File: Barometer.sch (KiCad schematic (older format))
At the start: 5 parts, among them U9 BMP388

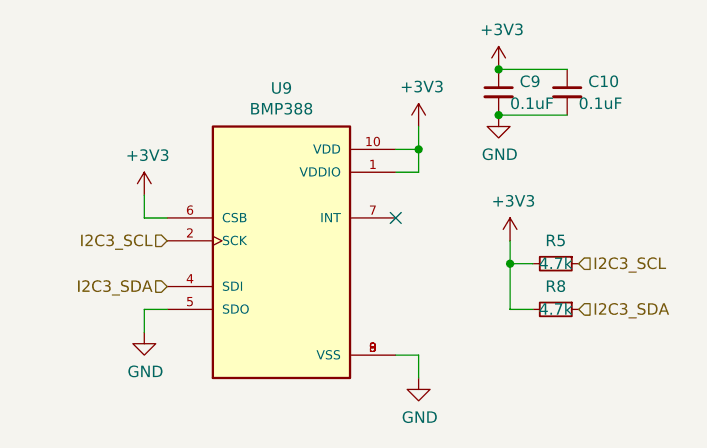
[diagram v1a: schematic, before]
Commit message: Changes made
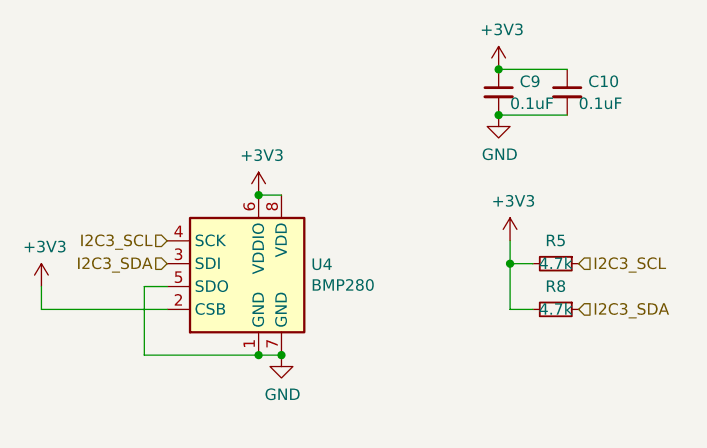
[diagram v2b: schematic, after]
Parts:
- removed U9: BMP388, Footprints:BMP388, symbol JPW_Symbols:BMP388
- added U4: BMP280, Package_LGA:Bosch_LGA-8_2x2.5mm_P0.65mm_ClockwisePinNumbering, symbol Sensor_Pressure:BMP280
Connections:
- net +3V3: now also U4.2 (CSB), U4.6 (VDDIO), U4.8 (VDD)
- net GND: now also U4.1 (GND), U4.5 (SDO), U4.7 (GND)
- net I2C3_SCL: now also U4.4 (SCK)
- net I2C3_SDA: now also U4.3 (SDI)
- no-connect marks 1 -> 0
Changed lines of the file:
@@
 $Descr A4 11693 8268
 encoding utf-8
-Sheet 7 7
+Sheet 5 7
 Title ""
 Date ""
@@
 Comment4 ""
 $EndDescr
-Text HLabel 5650 3950 0    50   Input ~ 0
+Text HLabel 5650 3850 0    50   Input ~ 0
 I2C3_SDA
 Text HLabel 5650 3750 0    50   Input ~ 0
 I2C3_SCL
 $Comp
-L JPW_Symbols:BMP388 U9
-U 1 1 608E517F
-P 6150 3850
-F 0 "U9" H 6150 4617 50  0000 C CNN
-F 1 "BMP388" H 6150 4526 50  0000 C CNN
-F 2 "Footprints:BMP388" H 6150 4600 50  0001 L BNN
-F 3 "" H 6150 3850 50  0001 L BNN
-	1    6150 3850
+L power:+3V3 #PWR0110
+U 1 1 608E9117
+P 6050 3550
+F 0 "#PWR0110" H 6050 3400 50  0001 C CNN
+F 1 "+3V3" H 6065 3723 50  0000 C CNN
+F 2 "" H 6050 3550 50  0001 C CNN
+F 3 "" H 6050 3550 50  0001 C CNN
+	1    6050 3550
 	1    0    0    -1
 $EndComp
 $Comp
-L power:+3V3 #PWR0110
-U 1 1 608E9117
-P 6750 3250
-F 0 "#PWR0110" H 6750 3100 50  0001 C CNN
-F 1 "+3V3" H 6765 3423 50  0000 C CNN
-F 2 "" H 6750 3250 50  0001 C CNN
-F 3 "" H 6750 3250 50  0001 C CNN
-	1    6750 3250
+L power:GND #PWR0171
+U 1 1 608EAE19
+P 6150 4250
+F 0 "#PWR0171" H 6150 4000 50  0001 C CNN
+F 1 "GND" H 6155 4077 50  0000 C CNN
+F 2 "" H 6150 4250 50  0001 C CNN
+F 3 "" H 6150 4250 50  0001 C CNN
+	1    6150 4250
 	1    0    0    -1
 $EndComp
 Wire Wire Line
-	6650 3350 6750 3350
-Wire Wire Line
-	6750 3350 6750 3250
-Wire Wire Line
-	6750 3350 6750 3450
-Wire Wire Line
-	6750 3450 6650 3450
-Connection ~ 6750 3350
-$Comp
-L power:+3V3 #PWR0111
-U 1 1 608E9B71
-P 5550 3550
-F 0 "#PWR0111" H 5550 3400 50  0001 C CNN
-F 1 "+3V3" H 5565 3723 50  0000 C CNN
-F 2 "" H 5550 3550 50  0001 C CNN
-F 3 "" H 5550 3550 50  0001 C CNN
-	1    5550 3550
-	1    0    0    -1
-$EndComp
-Wire Wire Line
-	5550 3550 5550 3650
-Wire Wire Line
-	5550 3650 5650 3650
-$Comp
-L power:GND #PWR0170
-U 1 1 608EA4FC
-P 5550 4150
-F 0 "#PWR0170" H 5550 3900 50  0001 C CNN
-F 1 "GND" H 5555 3977 50  0000 C CNN
-F 2 "" H 5550 4150 50  0001 C CNN
-F 3 "" H 5550 4150 50  0001 C CNN
-	1    5550 4150
-	1    0    0    -1
-$EndComp
-Wire Wire Line
-	5550 4150 5550 4050
-Wire Wire Line
-	5550 4050 5650 4050
-$Comp
-L power:GND #PWR0171
-U 1 1 608EAE19
-P 6750 4350
-F 0 "#PWR0171" H 6750 4100 50  0001 C CNN
-F 1 "GND" H 6755 4177 50  0000 C CNN
-F 2 "" H 6750 4350 50  0001 C CNN
-F 3 "" H 6750 4350 50  0001 C CNN
-	1    6750 4350
-	1    0    0    -1
-$EndComp
-Wire Wire Line
-	6750 4350 6750 4250
-Wire Wire Line
-	6750 4250 6650 4250
-NoConn ~ 6650 3650
+	6150 4250 6050 4250
 $Comp
 L power:+3V3 #PWR0174
@@
 Wire Wire Line
 	7100 3000 7400 3000
-Connection ~ 7100 3000
 $Comp
 L power:GND #PWR0176
@@
 	1    0    0    -1
 $EndComp
-Connection ~ 7100 3200
 Wire Wire Line
 	7100 3200 7400 3200
+$Comp
+L Sensor_Pressure:BMP280 U4
+U 1 1 60D6237A
+P 6050 3950
+F 0 "U4" H 6280 4046 50  0000 L CNN
+F 1 "BMP280" H 6280 3955 50  0000 L CNN
+F 2 "Package_LGA:Bosch_LGA-8_2x2.5mm_P0.65mm_ClockwisePinNumbering" H 6050 3250 50  0001 C CNN
+F 3 "https://ae-bst.resource.bosch.com/media/_tech/media/datasheets/BST-BMP280-DS001.pdf" H 6050 3950 50  0001 C CNN
+	1    6050 3950
+	1    0    0    -1
+$EndComp
+Connection ~ 6150 4250
+Wire Wire Line
+	6050 3550 6150 3550
+Connection ~ 6050 3550
+Wire Wire Line
+	5650 3950 5550 3950
+Wire Wire Line
+	5550 3950 5550 4250
+Wire Wire Line
+	5550 4250 6050 4250
+Connection ~ 6050 4250
+$Comp
+L power:+3V3 #PWR0103
+U 1 1 60D6B9F1
+P 5100 3950
+F 0 "#PWR0103" H 5100 3800 50  0001 C CNN
+F 1 "+3V3" H 5115 4123 50  0000 C CNN
+F 2 "" H 5100 3950 50  0001 C CNN
+F 3 "" H 5100 3950 50  0001 C CNN
+	1    5100 3950
+	1    0    0    -1
+$EndComp
+Wire Wire Line
+	5100 3950 5100 4050
+Wire Wire Line
+	5100 4050 5650 4050
+Connection ~ 7100 3000
+Connection ~ 7100 3200
 $EndSCHEMATC
